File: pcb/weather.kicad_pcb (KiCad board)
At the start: 2 copper layers, 50 x 75 mm, 27 parts, among them J1 dht11, J2 EXTRA PINS, J3 Conn_01x02_Pin, U2 TFT_ST7735_SD, U3 WEMOS_C3_Mini

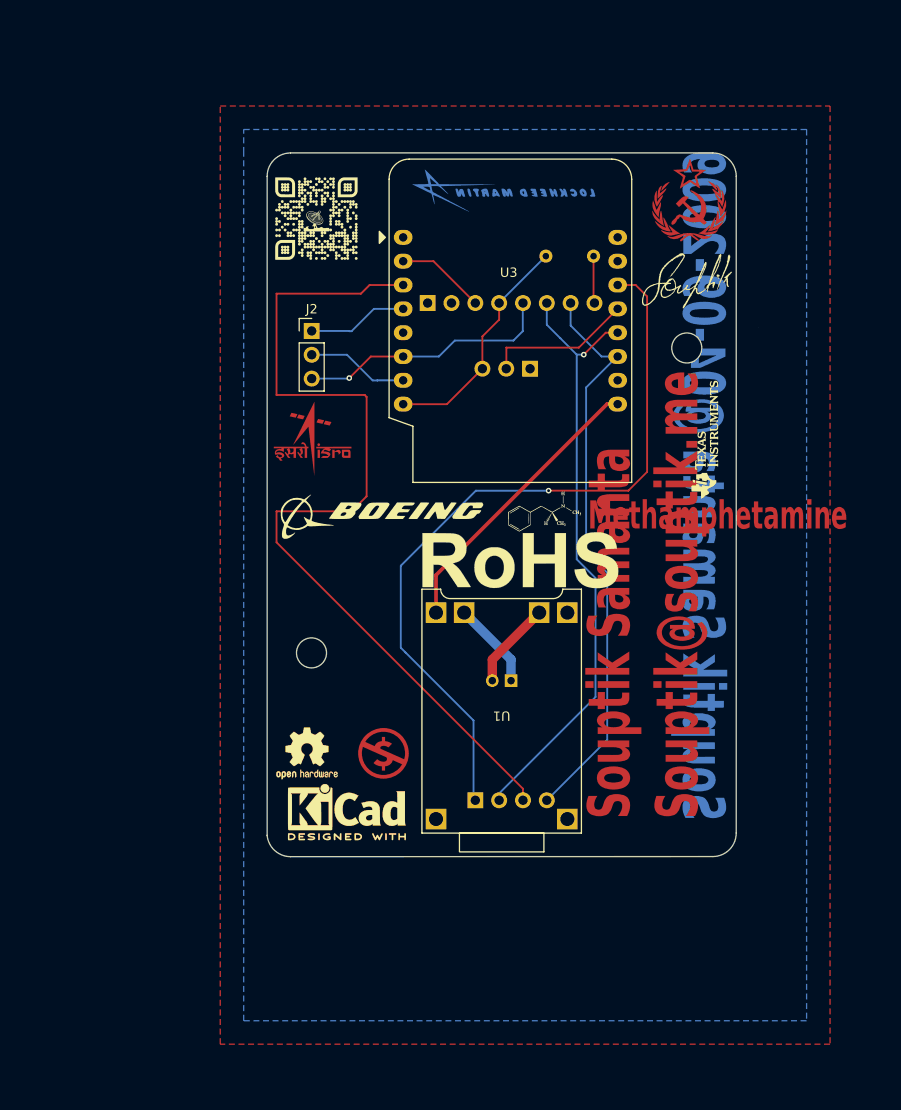
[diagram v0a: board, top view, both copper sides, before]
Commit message: Add files via upload
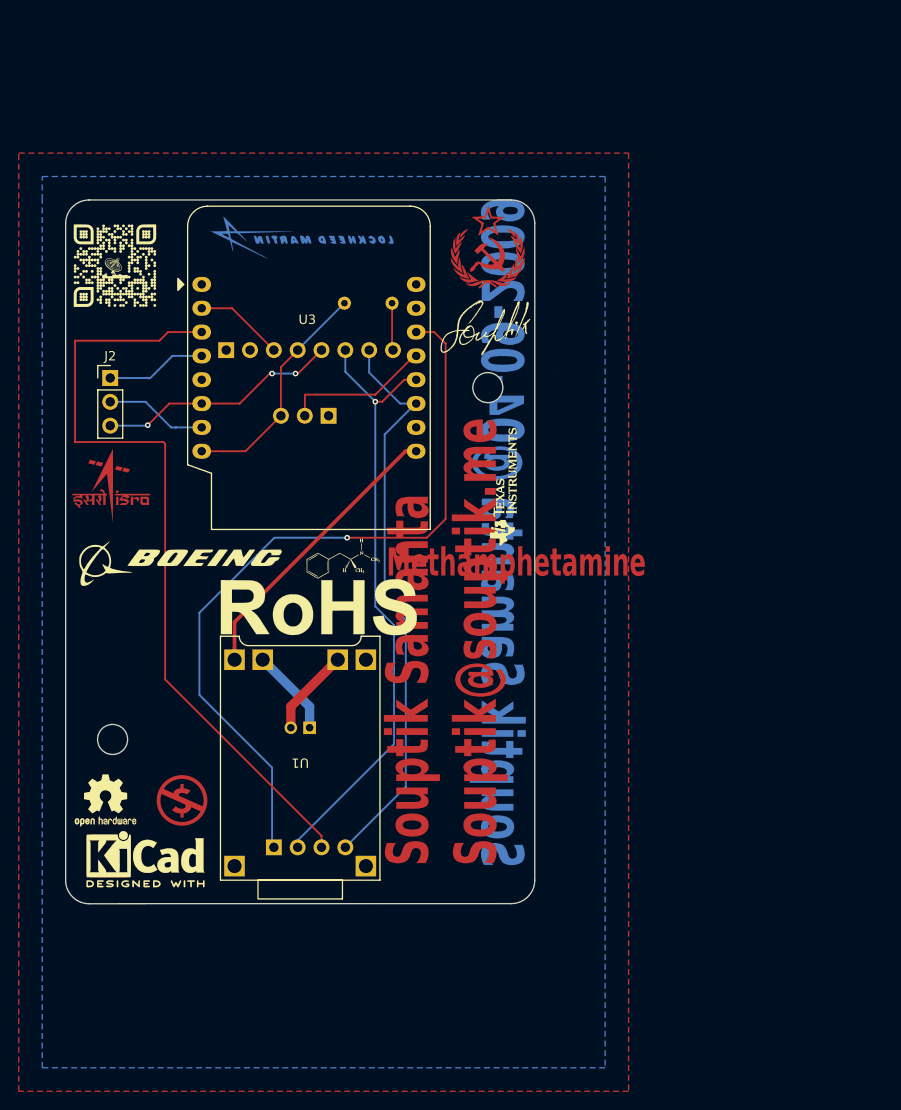
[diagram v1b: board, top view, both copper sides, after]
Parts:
- moved REF** 23.1 mm to (152.5, 87.5)
- moved G*** 22.1 mm to (152.5, 60.8) (x2)
- moved G*** 22.1 mm to (172.7, 34.4) (x2)
- moved G*** 22.1 mm to (194.1, 43.8)
- moved G*** 22.1 mm to (192.5, 35.4) (x2)
- moved G*** 22.1 mm to (159.7, 68.4)
- moved G*** 22.1 mm to (177.1, 68.2)
- moved G*** 22.1 mm to (194.1, 60.6)
- moved G*** 22.1 mm to (152.8, 37.0)
- moved J2 22.1 mm to (152.2, 49.0)
- moved J3 22.1 mm to (173.5, 86.2)
- moved REF** 22.1 mm to (151.8, 94.0)
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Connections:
- U2 pad 1: unconnected-(U2-3V3-Pad1) -> VCC
- U2 pad 2: unconnected-(U2-GND-Pad2) -> GND
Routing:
- net MISO: track 96.9 -> 84.3 mm
- net IO4: track 27.6 -> 25.9 mm, vias 1 -> 3
